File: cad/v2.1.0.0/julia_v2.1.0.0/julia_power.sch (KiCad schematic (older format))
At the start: 47 parts, among them J1 Barrel_Jack_Switch, U2 AZ1117-3.3, U3 AZ1117-2.5, U4 NCP565ST12T3G

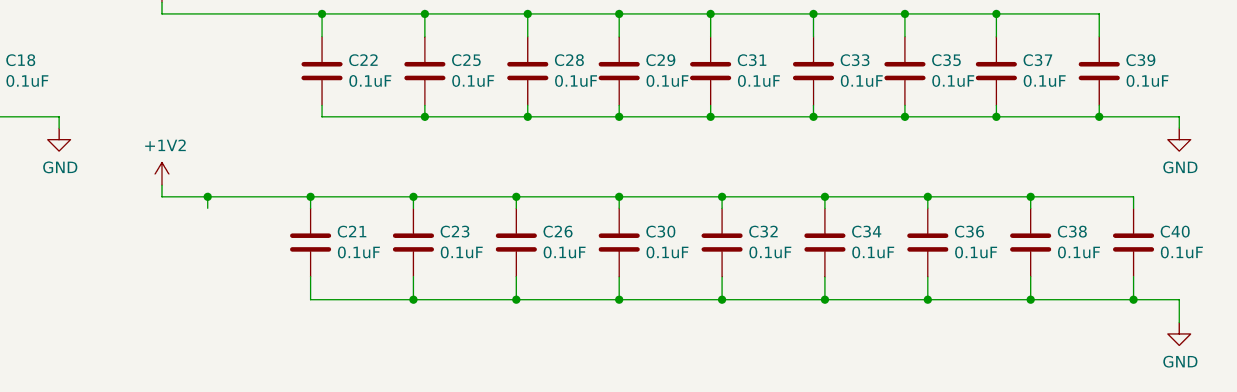
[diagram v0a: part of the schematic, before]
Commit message: Layout complete(?)
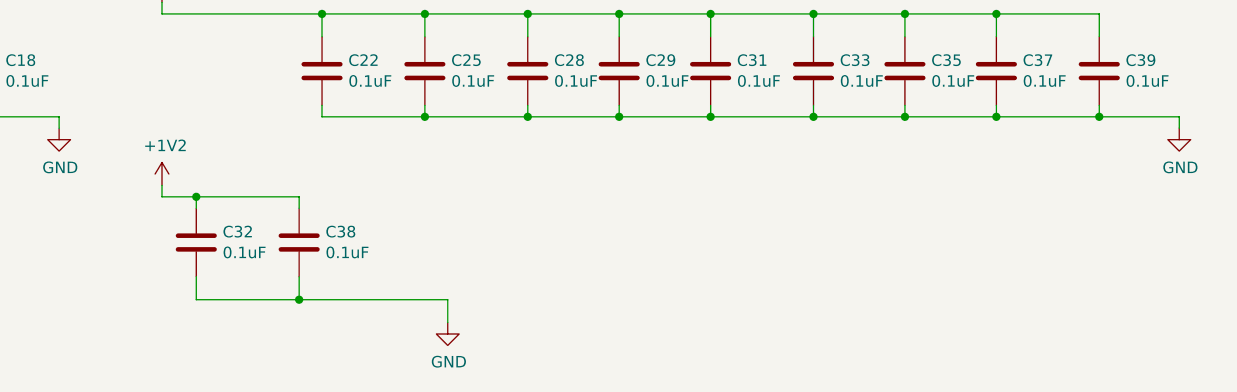
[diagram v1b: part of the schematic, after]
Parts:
- removed C21, C23, C26, C30, C34, C36, C40: 0.1uF, Capacitor_SMD:C_0402_1005Metric, symbol Device:C
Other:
- moved on the sheet: C32, C38
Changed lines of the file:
@@
 $EndComp
 Wire Wire Line
-	9850 6000 9400 6000
-Connection ~ 9850 6000
-Wire Wire Line
-	9850 5900 9850 6000
-Wire Wire Line
-	9400 6000 8950 6000
-Connection ~ 9400 6000
-Wire Wire Line
-	9400 5900 9400 6000
-Wire Wire Line
-	8950 6000 8500 6000
-Connection ~ 8950 6000
-Wire Wire Line
-	8950 5900 8950 6000
-Wire Wire Line
-	8500 6000 8050 6000
-Connection ~ 8500 6000
-Wire Wire Line
-	8500 5900 8500 6000
-Wire Wire Line
-	8050 6000 7600 6000
-Connection ~ 8050 6000
-Wire Wire Line
-	8050 5900 8050 6000
-Wire Wire Line
-	7600 6000 7150 6000
-Connection ~ 7600 6000
-Wire Wire Line
-	7600 5900 7600 6000
-Wire Wire Line
-	7150 6000 6700 6000
-Connection ~ 7150 6000
-Wire Wire Line
-	7150 5900 7150 6000
-Wire Wire Line
-	6700 6000 6250 6000
-Connection ~ 6700 6000
-Wire Wire Line
-	6700 5900 6700 6000
-Wire Wire Line
-	6250 5900 6250 6000
-Wire Wire Line
-	8500 5550 8950 5550
-Connection ~ 8500 5550
-Wire Wire Line
-	8500 5600 8500 5550
-Wire Wire Line
-	8950 5550 9400 5550
-Connection ~ 8950 5550
-Wire Wire Line
-	8950 5600 8950 5550
-Wire Wire Line
-	9400 5550 9850 5550
-Connection ~ 9400 5550
-Wire Wire Line
-	9400 5600 9400 5550
-Wire Wire Line
-	8050 5550 8500 5550
-Connection ~ 8050 5550
-Wire Wire Line
-	8050 5600 8050 5550
-Wire Wire Line
-	7600 5550 8050 5550
-Connection ~ 7600 5550
-Wire Wire Line
-	7600 5600 7600 5550
-Wire Wire Line
-	7150 5550 7600 5550
-Connection ~ 7150 5550
-Wire Wire Line
-	7150 5600 7150 5550
-Wire Wire Line
-	6700 5550 7150 5550
-Connection ~ 6700 5550
-Wire Wire Line
-	6700 5600 6700 5550
-Wire Wire Line
-	6250 5550 6700 5550
-Connection ~ 6250 5550
-Wire Wire Line
-	6250 5600 6250 5550
-Wire Wire Line
-	5800 5550 6250 5550
-Connection ~ 5800 5550
-Wire Wire Line
-	5800 5600 5800 5550
-Wire Wire Line
-	10050 6000 9850 6000
-Wire Wire Line
-	10050 6100 10050 6000
-Wire Wire Line
-	9850 5550 9850 5600
-Wire Wire Line
-	5600 5550 5800 5550
+	6200 5900 6200 6000
+Wire Wire Line
+	5750 5900 5750 6000
+Wire Wire Line
+	6200 5600 6200 5550
+Wire Wire Line
+	5750 5600 5750 5550
+Wire Wire Line
+	6850 6100 6850 6000
 Wire Wire Line
 	5600 5500 5600 5550
@@
 L power:GND #PWR0117
 U 1 1 6020D2AD
-P 10050 6100
-F 0 "#PWR0117" H 10050 5850 50  0001 C CNN
-F 1 "GND" H 10055 5927 50  0000 C CNN
-F 2 "" H 10050 6100 50  0001 C CNN
-F 3 "" H 10050 6100 50  0001 C CNN
-	1    10050 6100
-	1    0    0    -1
-$EndComp
-$Comp
-L Device:C C40
-U 1 1 6020CCFB
-P 9850 5750
-F 0 "C40" H 9965 5796 50  0000 L CNN
-F 1 "0.1uF" H 9965 5705 50  0000 L CNN
-F 2 "Capacitor_SMD:C_0402_1005Metric" H 9888 5600 50  0001 C CNN
-F 3 "~" H 9850 5750 50  0001 C CNN
-	1    9850 5750
+P 6850 6100
+F 0 "#PWR0117" H 6850 5850 50  0001 C CNN
+F 1 "GND" H 6855 5927 50  0000 C CNN
+F 2 "" H 6850 6100 50  0001 C CNN
+F 3 "" H 6850 6100 50  0001 C CNN
+	1    6850 6100
 	1    0    0    -1
 $EndComp
@@
 L Device:C C38
 U 1 1 6020C7C1
-P 9400 5750
-F 0 "C38" H 9515 5796 50  0000 L CNN
-F 1 "0.1uF" H 9515 5705 50  0000 L CNN
-F 2 "Capacitor_SMD:C_0402_1005Metric" H 9438 5600 50  0001 C CNN
-F 3 "~" H 9400 5750 50  0001 C CNN
-	1    9400 5750
-	1    0    0    -1
-$EndComp
-$Comp
-L Device:C C36
-U 1 1 6020C1D4
-P 8950 5750
-F 0 "C36" H 9065 5796 50  0000 L CNN
-F 1 "0.1uF" H 9065 5705 50  0000 L CNN
-F 2 "Capacitor_SMD:C_0402_1005Metric" H 8988 5600 50  0001 C CNN
-F 3 "~" H 8950 5750 50  0001 C CNN
-	1    8950 5750
-	1    0    0    -1
-$EndComp
-$Comp
-L Device:C C34
-U 1 1 6020BC15
-P 8500 5750
-F 0 "C34" H 8615 5796 50  0000 L CNN
-F 1 "0.1uF" H 8615 5705 50  0000 L CNN
-F 2 "Capacitor_SMD:C_0402_1005Metric" H 8538 5600 50  0001 C CNN
-F 3 "~" H 8500 5750 50  0001 C CNN
-	1    8500 5750
+P 6200 5750
+F 0 "C38" H 6315 5796 50  0000 L CNN
+F 1 "0.1uF" H 6315 5705 50  0000 L CNN
+F 2 "Capacitor_SMD:C_0402_1005Metric" H 6238 5600 50  0001 C CNN
+F 3 "~" H 6200 5750 50  0001 C CNN
+	1    6200 5750
 	1    0    0    -1
 $EndComp
@@
 L Device:C C32
 U 1 1 6020B6A5
-P 8050 5750
-F 0 "C32" H 8165 5796 50  0000 L CNN
-F 1 "0.1uF" H 8165 5705 50  0000 L CNN
-F 2 "Capacitor_SMD:C_0402_1005Metric" H 8088 5600 50  0001 C CNN
-F 3 "~" H 8050 5750 50  0001 C CNN
-	1    8050 5750
-	1    0    0    -1
-$EndComp
-$Comp
-L Device:C C30
-U 1 1 6020B1E8
-P 7600 5750
-F 0 "C30" H 7715 5796 50  0000 L CNN
-F 1 "0.1uF" H 7715 5705 50  0000 L CNN
-F 2 "Capacitor_SMD:C_0402_1005Metric" H 7638 5600 50  0001 C CNN
-F 3 "~" H 7600 5750 50  0001 C CNN
-	1    7600 5750
-	1    0    0    -1
-$EndComp
-$Comp
-L Device:C C26
-U 1 1 6020ACC7
-P 7150 5750
-F 0 "C26" H 7265 5796 50  0000 L CNN
-F 1 "0.1uF" H 7265 5705 50  0000 L CNN
-F 2 "Capacitor_SMD:C_0402_1005Metric" H 7188 5600 50  0001 C CNN
-F 3 "~" H 7150 5750 50  0001 C CNN
-	1    7150 5750
-	1    0    0    -1
-$EndComp
-$Comp
-L Device:C C23
-U 1 1 6020A7B8
-P 6700 5750
-F 0 "C23" H 6815 5796 50  0000 L CNN
-F 1 "0.1uF" H 6815 5705 50  0000 L CNN
-F 2 "Capacitor_SMD:C_0402_1005Metric" H 6738 5600 50  0001 C CNN
-F 3 "~" H 6700 5750 50  0001 C CNN
-	1    6700 5750
-	1    0    0    -1
-$EndComp
-$Comp
-L Device:C C21
-U 1 1 6020A22E
-P 6250 5750
-F 0 "C21" H 6365 5796 50  0000 L CNN
-F 1 "0.1uF" H 6365 5705 50  0000 L CNN
-F 2 "Capacitor_SMD:C_0402_1005Metric" H 6288 5600 50  0001 C CNN
-F 3 "~" H 6250 5750 50  0001 C CNN
-	1    6250 5750
+P 5750 5750
+F 0 "C32" H 5865 5796 50  0000 L CNN
+F 1 "0.1uF" H 5865 5705 50  0000 L CNN
+F 2 "Capacitor_SMD:C_0402_1005Metric" H 5788 5600 50  0001 C CNN
+F 3 "~" H 5750 5750 50  0001 C CNN
+	1    5750 5750
 	1    0    0    -1
 $EndComp
@@
 Wire Wire Line
 	5600 4750 6300 4750
+Wire Wire Line
+	6200 6000 6850 6000
+Wire Wire Line
+	5600 5550 5750 5550
+Wire Wire Line
+	6200 5550 5750 5550
+Connection ~ 5750 5550
+Wire Wire Line
+	5750 6000 6200 6000
+Connection ~ 6200 6000
 $EndSCHEMATC
